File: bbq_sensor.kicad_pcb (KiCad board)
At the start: 2 copper layers, 25.5 x 30 mm, 3 parts, among them J1 Conn_01x06_Socket, P1 Connector_Generic:Conn_01x08, P2 Connector_Generic:Conn_01x08

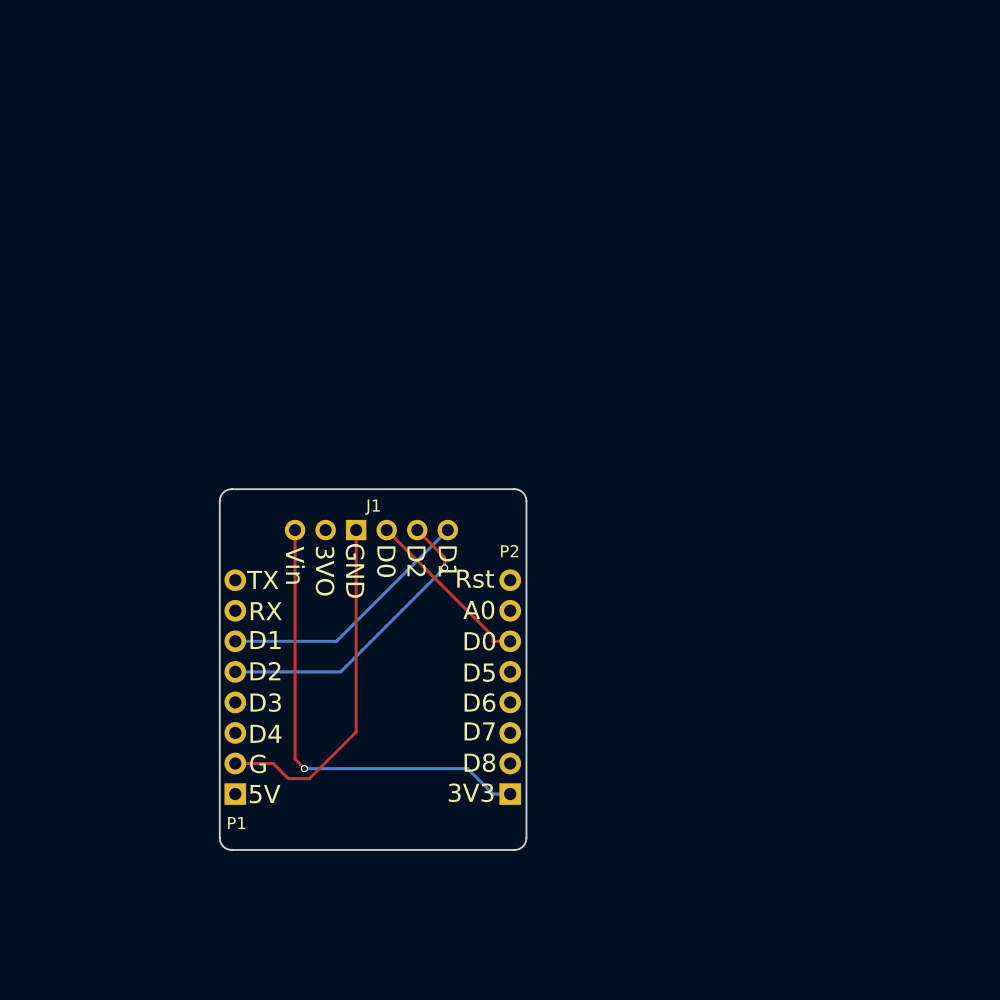
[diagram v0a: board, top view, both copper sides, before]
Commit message: improved pcb
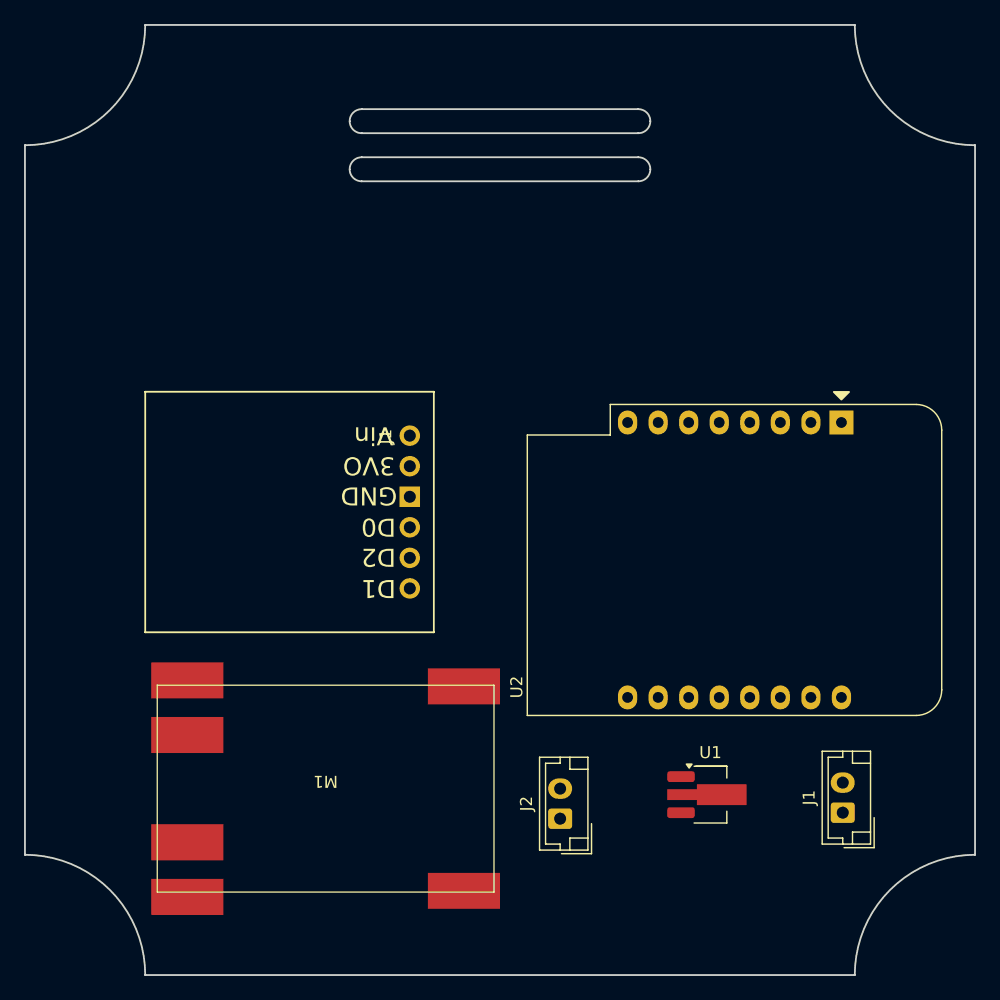
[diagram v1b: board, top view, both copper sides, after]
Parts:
- removed P1, P2: Connector_Generic:Conn_01x08, D1_mini:D1_mini_Pin_Header
- added J1: Conn_01x02_Socket, Connector_JST:JST_EH_B2B-EH-A_1x02_P2.50mm_Vertical, F.Cu at (178.0, 105.5)
- added J2: Conn_01x02_Socket, Connector_JST:JST_EH_B2B-EH-A_1x02_P2.50mm_Vertical, F.Cu at (154.5, 106.0)
- added M1: ~, tp4056-module:tp4056-module, F.Cu at (149.0, 94.9)
- added U1: LM1117DT-3.3, Package_TO_SOT_SMD:SOT-89-3_Handsoldering, F.Cu at (167.0, 104.0)
- added U2: WEMOS_D1_mini, RF_Module:WEMOS_D1_mini_light, F.Cu at (177.9, 73.1)
- moved J1 12.4 mm to (142.0, 74.2), turned to 0 degrees
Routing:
- net /+3.3V: track 38.1 -> 0.00 mm, vias 1 -> 0
- net /GND: track 29.0 -> 0.00 mm
- net /D2: track 25.1 -> 0.00 mm, vias 1 -> 0
- net /D1: track 21.5 -> 0.00 mm
- net /D0: track 14.3 -> 0.00 mm
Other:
- board size 25.5 x 30 mm -> 79 x 79 mm
- board text removed: "3V3"
- board text removed: "5V"
- board text removed: "A0"
- board text removed: "D3"
- board text removed: "D4"
- board text removed: "D5"
- board text removed: "D6"
- board text removed: "D7"
- board text removed: "D8"
- board text removed: "G"
- board text removed: "RX"
- board text removed: "Rst"
- board text removed: "TX"
